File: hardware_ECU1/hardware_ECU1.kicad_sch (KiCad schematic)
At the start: 17 parts, among them J1 Micro_SD_Card, U1 step-down (buck), U2 MPU-6050, U3 ESP32-WROOM-32

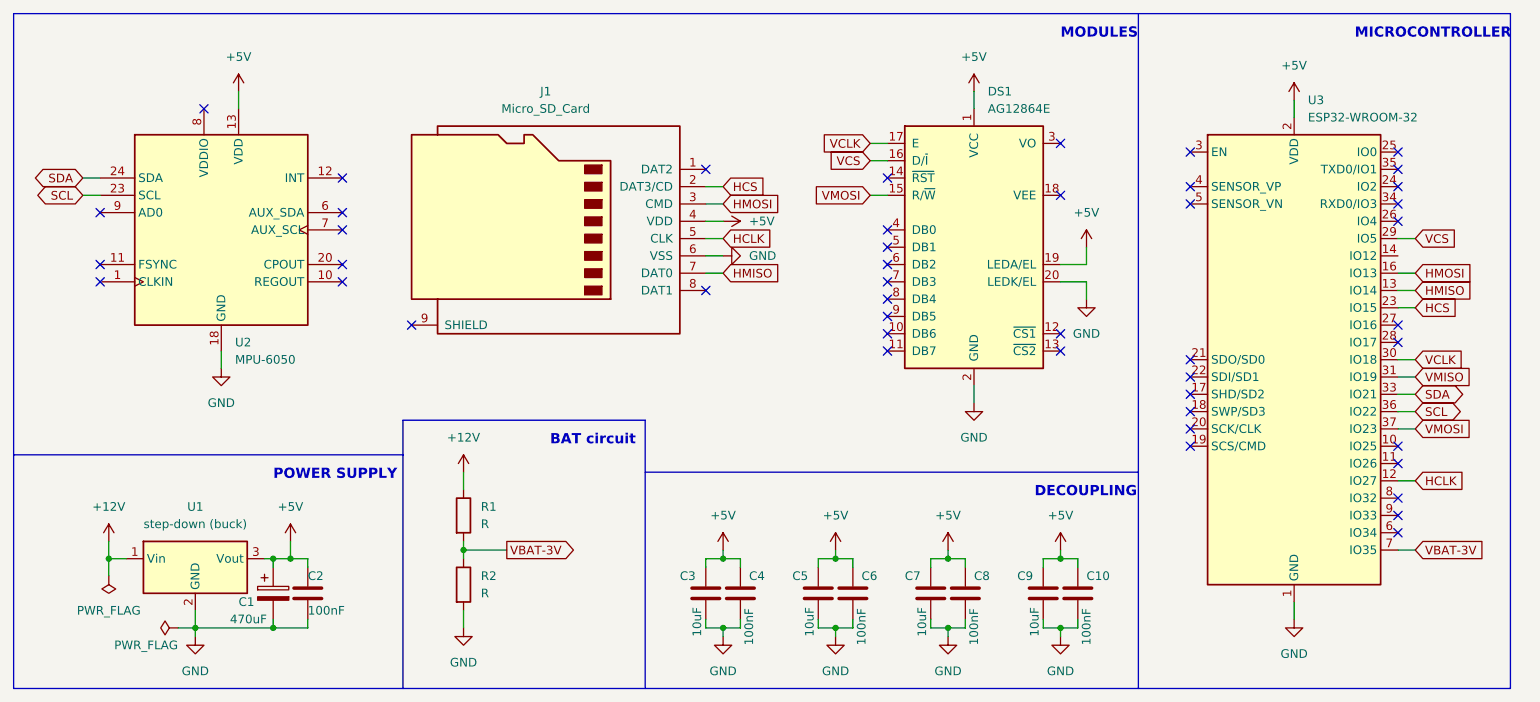
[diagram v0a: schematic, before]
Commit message: Update hardware_ECU1.kicad_sch
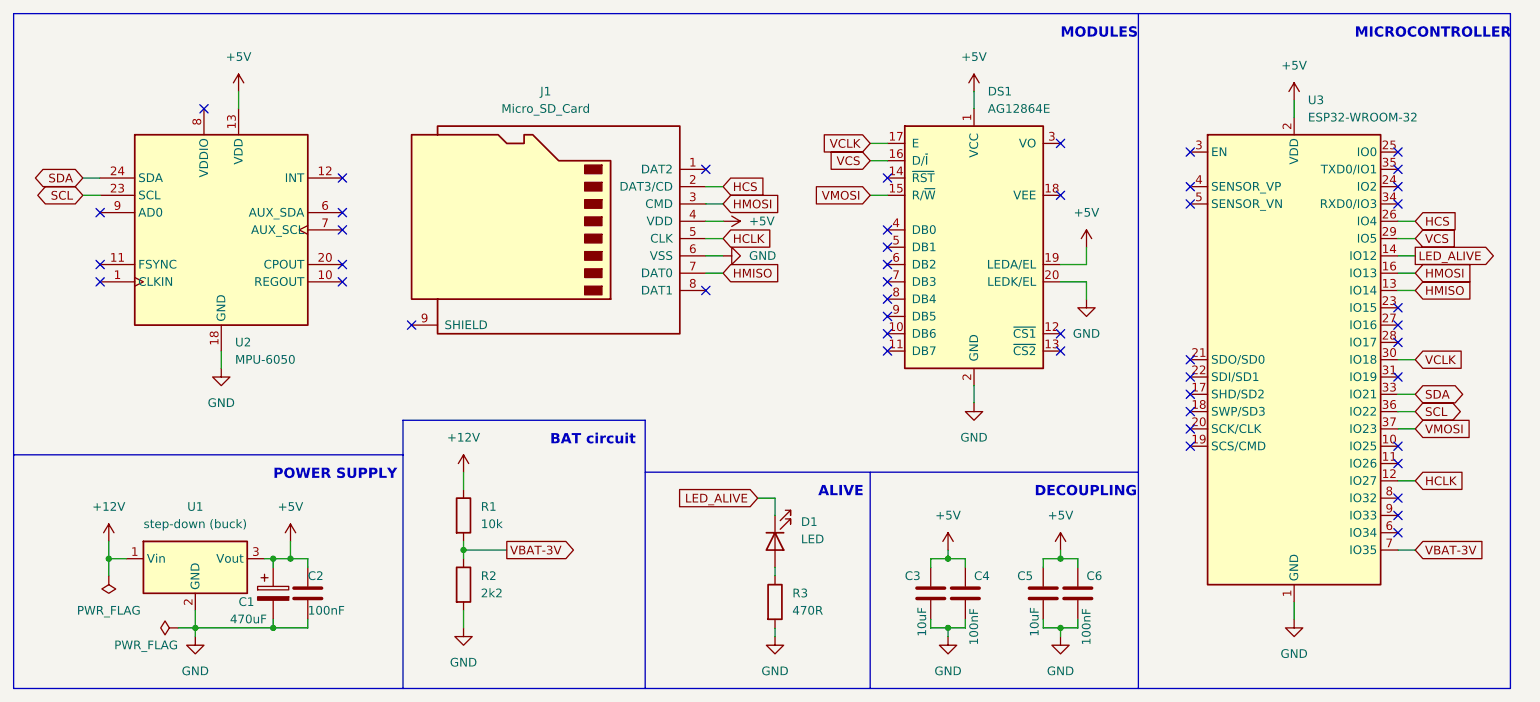
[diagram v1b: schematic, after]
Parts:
- removed C3, C5: 10uF, symbol Device:C
- removed C4, C6: 100nF, symbol Device:C
- added D1: LED, symbol Device:LED
- added R3: 470R, symbol Device:R
- R1: value R -> 10k
- R2: value R -> 2k2
- renumbered C7 to C3, C8 to C4, C9 to C5, C10 to C6
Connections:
- net GND: now also R3.2
- net HCS: now also U3.26 (IO4); no longer U3.23 (IO15)
- net LED_ALIVE: now reaches U3.14 (IO12)
- net LED_ALIVE: now also D1.1 (K)
- net VMISO: no longer names the net of U3.31 (IO19)
- new net: D1.2 (A), R3.1
- no-connect marks 46 -> 47
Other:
- note added: "ALIVE"
